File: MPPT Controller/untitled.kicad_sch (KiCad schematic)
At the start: 32 parts, among them J5 USB_C_Receptacle_USB2.0_16P, J9 Conn_01x02_Pin, U2 ESP32-WROOM-32D, U3 CH340C

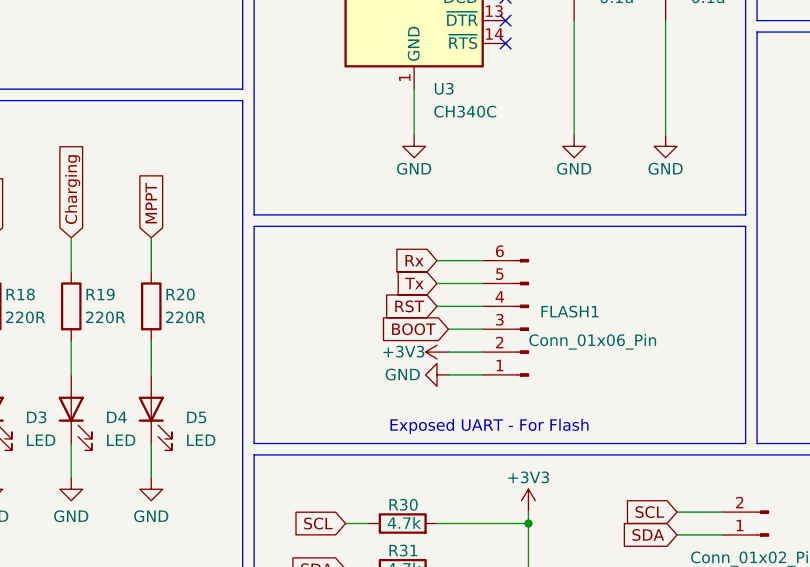
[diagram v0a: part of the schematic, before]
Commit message: Changes
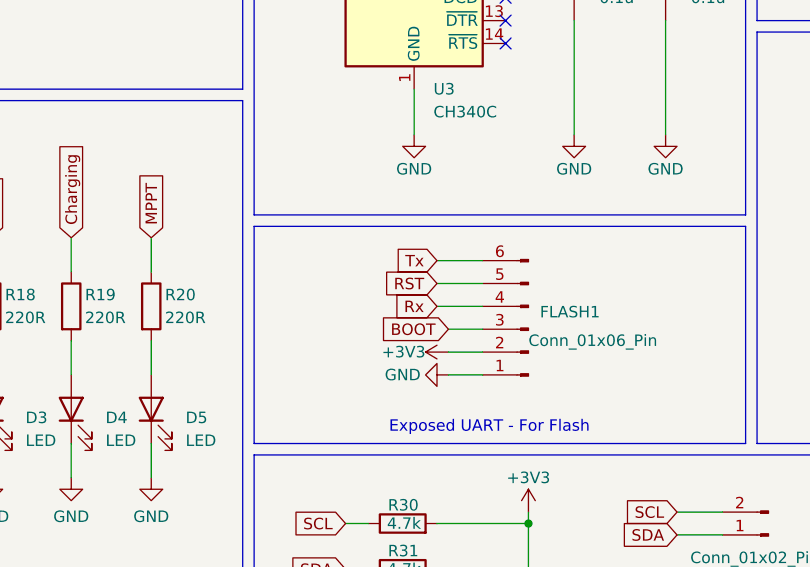
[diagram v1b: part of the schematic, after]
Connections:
- net RST: now also FLASH1.5 (Pin_5); no longer FLASH1.4 (Pin_4)
- net Rx: now also FLASH1.4 (Pin_4); no longer FLASH1.6 (Pin_6)
- net Tx: now also FLASH1.6 (Pin_6); no longer FLASH1.5 (Pin_5)

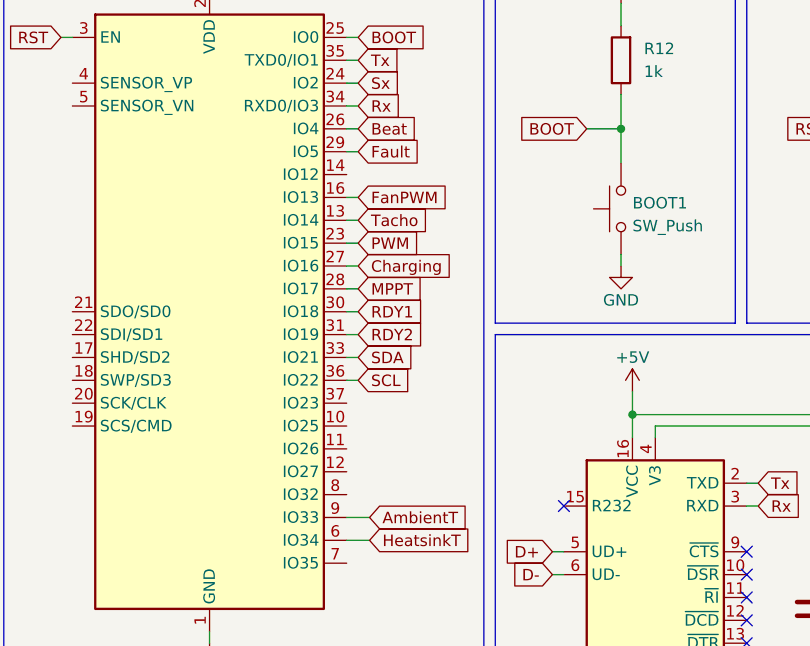
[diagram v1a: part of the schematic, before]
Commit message: DRC Run
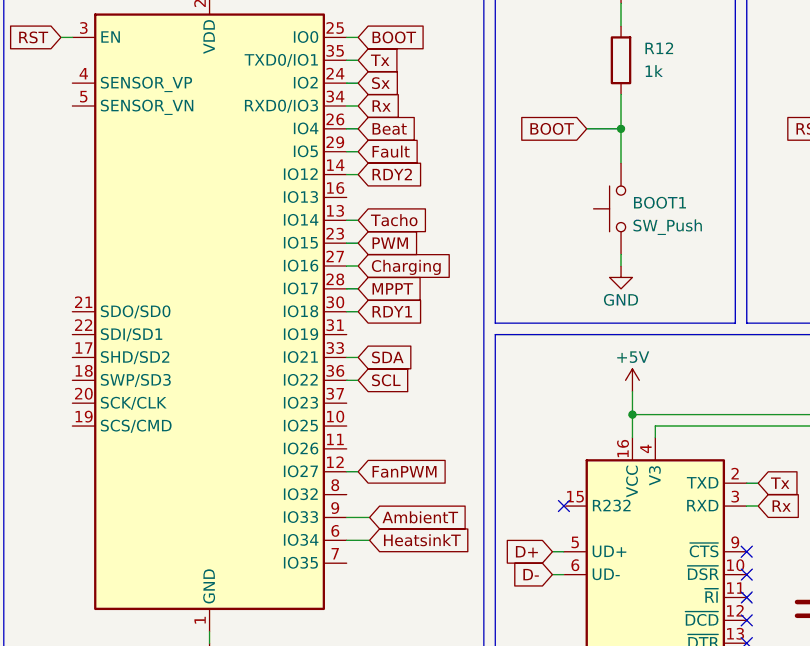
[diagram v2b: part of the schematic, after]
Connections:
- net FanPWM: now also U2.12 (IO27); no longer U2.16 (IO13)
- net RDY2: now also U2.14 (IO12); no longer U2.31 (IO19)
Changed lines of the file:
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@@
-	(wire
-		(pts
-			(xy 50.8 58.42) (xy 52.07 58.42)
-		)
-		(stroke
-			(width 0)
-			(type default)
-		)
-	)
 	(wire
 		(pts
@@
 	(wire
 		(pts
+			(xy 50.8 40.64) (xy 52.07 40.64)
+		)
+		(stroke
+			(width 0)
+			(type default)
+		)
+	)
+	(wire
+		(pts
 			(xy 142.24 60.96) (xy 142.24 76.2)
 		)
@@
 	(wire
 		(pts
-			(xy 50.8 43.18) (xy 52.07 43.18)
-		)
-		(stroke
-			(width 0)
-			(type default)
-		)
-	)
-	(wire
-		(pts
 			(xy 85.09 100.33) (xy 85.09 105.41)
 		)
@@
 	(wire
 		(pts
+			(xy 50.8 73.66) (xy 52.07 73.66)
+		)
+		(stroke
+			(width 0)
+			(type default)
+		)
+	)
+	(wire
+		(pts
 			(xy 113.03 67.31) (xy 82.55 67.31)
 		)
@@
 	(global_label "RDY2"
 		(shape input)
-		(at 52.07 58.42 0)
-		(fields_autoplaced yes)
-		(effects
-			(font
-				(size 1.27 1.27)
-			)
-			(justify left)
-		)
-		(property "Intersheetrefs" "${INTERSHEET_REFS}"
-			(at 59.8933 58.42 0)
+		(at 52.07 40.64 0)
+		(fields_autoplaced yes)
+		(effects
+			(font
+				(size 1.27 1.27)
+			)
+			(justify left)
+		)
+		(property "Intersheetrefs" "${INTERSHEET_REFS}"
+			(at 59.8933 40.64 0)
 			(effects
 				(font
@@
 	(global_label "FanPWM"
 		(shape input)
-		(at 52.07 43.18 0)
-		(fields_autoplaced yes)
-		(effects
-			(font
-				(size 1.27 1.27)
-			)
-			(justify left)
-		)
-		(property "Intersheetrefs" "${INTERSHEET_REFS}"
-			(at 62.6146 43.18 0)
-			(effects
-				(font
+		(at 52.07 73.66 0)
+		(fields_autoplaced yes)
+		(effects
+			(font
+				(size 1.27 1.27)
+			)
+			(justify left)
+		)
+		(property "Intersheetrefs" "${INTERSHEET_REFS}"
+			(at 62.6146 73.66 0)
+			(effects
+				(font

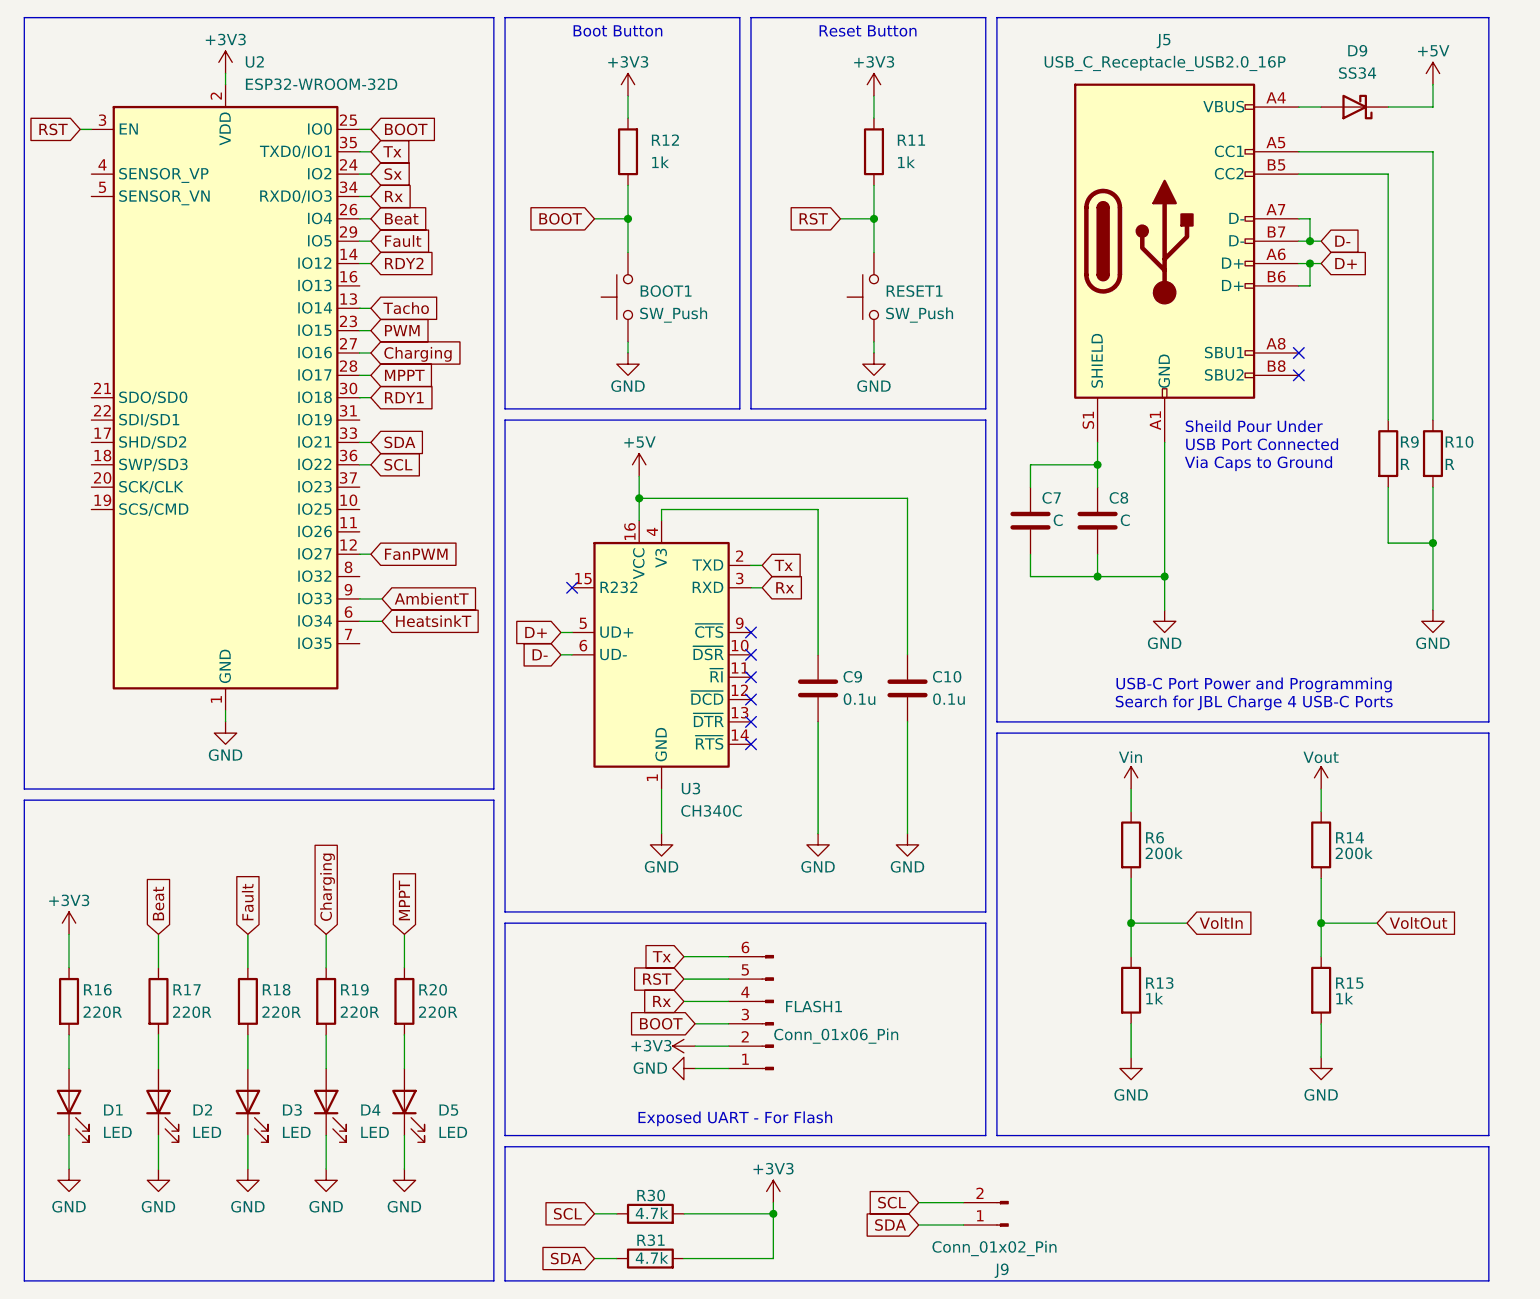
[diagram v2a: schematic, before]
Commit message: Logo
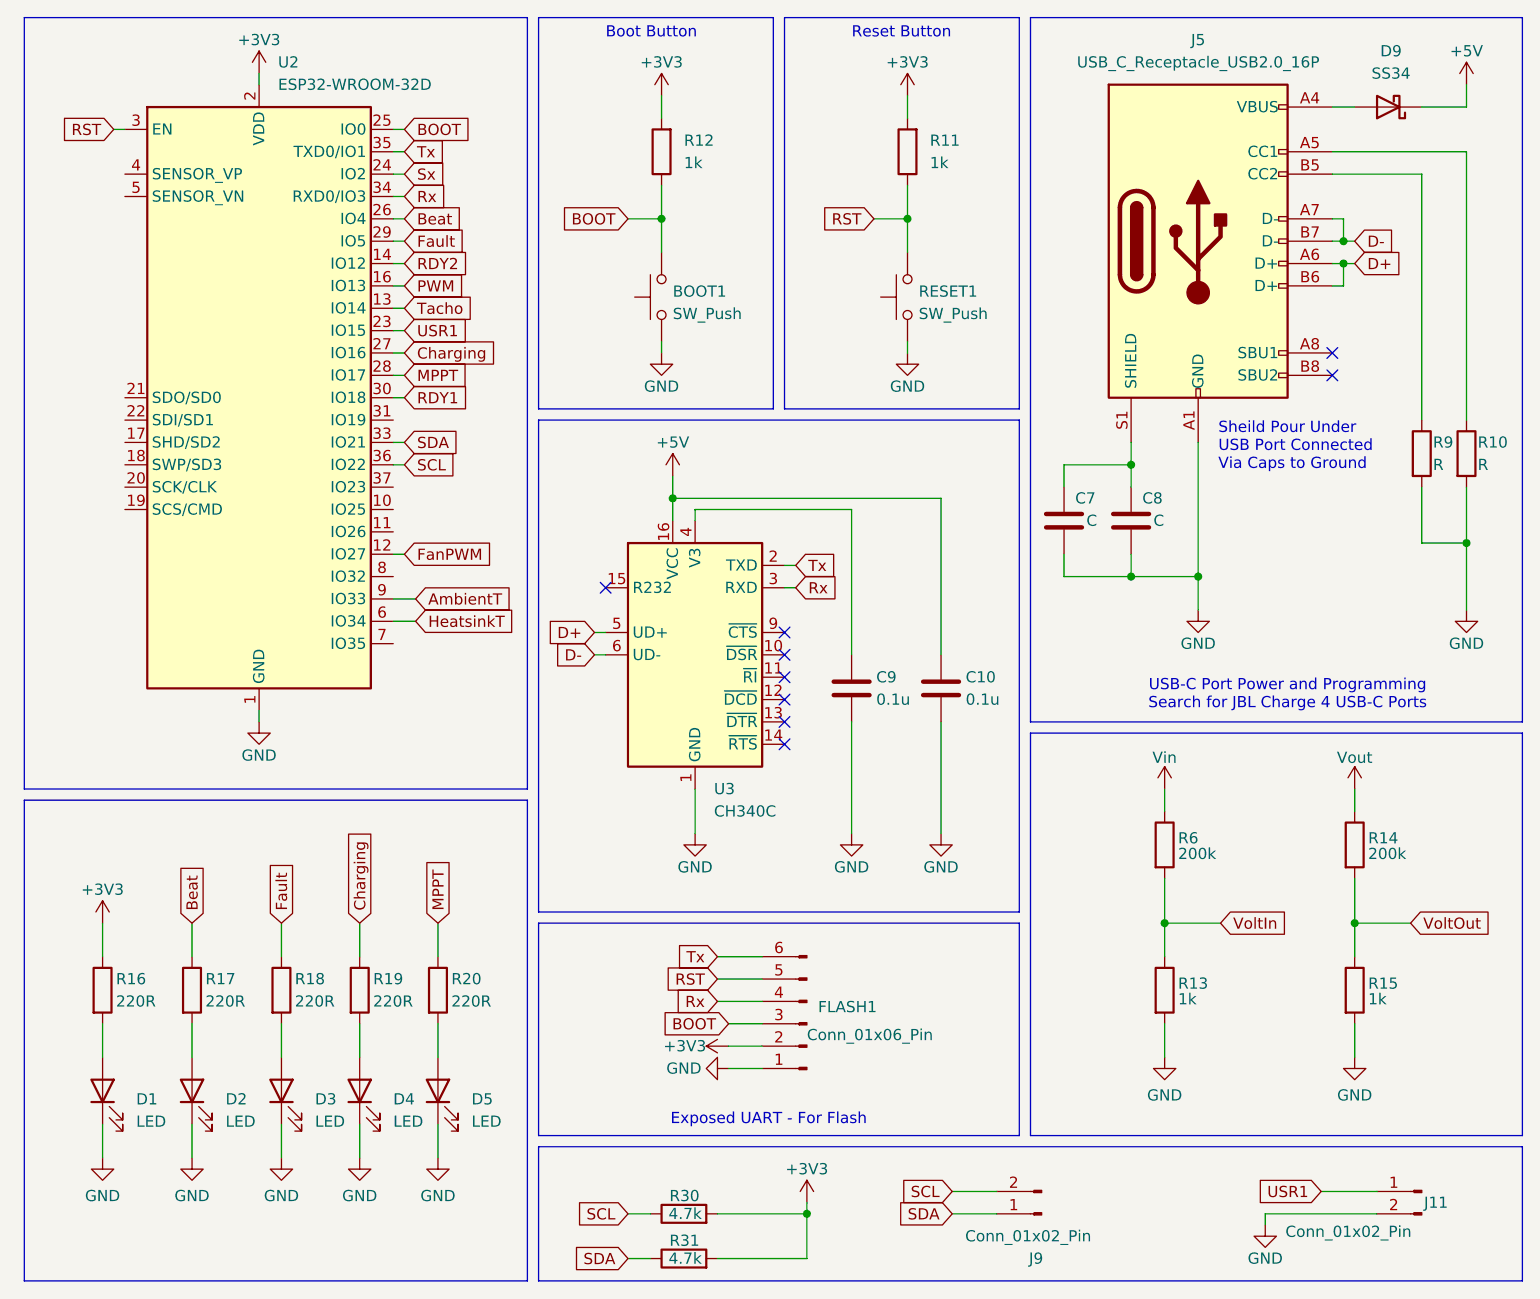
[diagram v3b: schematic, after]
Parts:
- added J11: Conn_01x02_Pin, Connector_PinSocket_2.54mm:PinSocket_2x01_P2.54mm_Vertical, symbol Connector:Conn_01x02_Pin
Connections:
- net GND: now also J11.2 (Pin_2)
- net PWM: now also U2.16 (IO13); no longer U2.23 (IO15)
- new net USR1: J11.1 (Pin_1), U2.23 (IO15)
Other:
- moved on the sheet: BOOT1, C10, C7, C8, C9, D1, D2, D3, D4, D5, D9, FLASH1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
